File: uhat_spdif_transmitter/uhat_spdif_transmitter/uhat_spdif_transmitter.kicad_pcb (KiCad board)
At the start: 2 copper layers, 65 x 30 mm, 75 parts, among them J1 GPIO_CONNECTOR, Q1 SS8050, SW1 SW_Push, U1 PLT131/T8, U10 USBLC6-2SC6, U2 LR8103A-T12, U4 W25Q32JVSSIQ, U5 24LC256T-I/SN, U6 PLT131/T8, U8 ICE40UP5K-SG48I, X1 1651-24575-BTBEYA

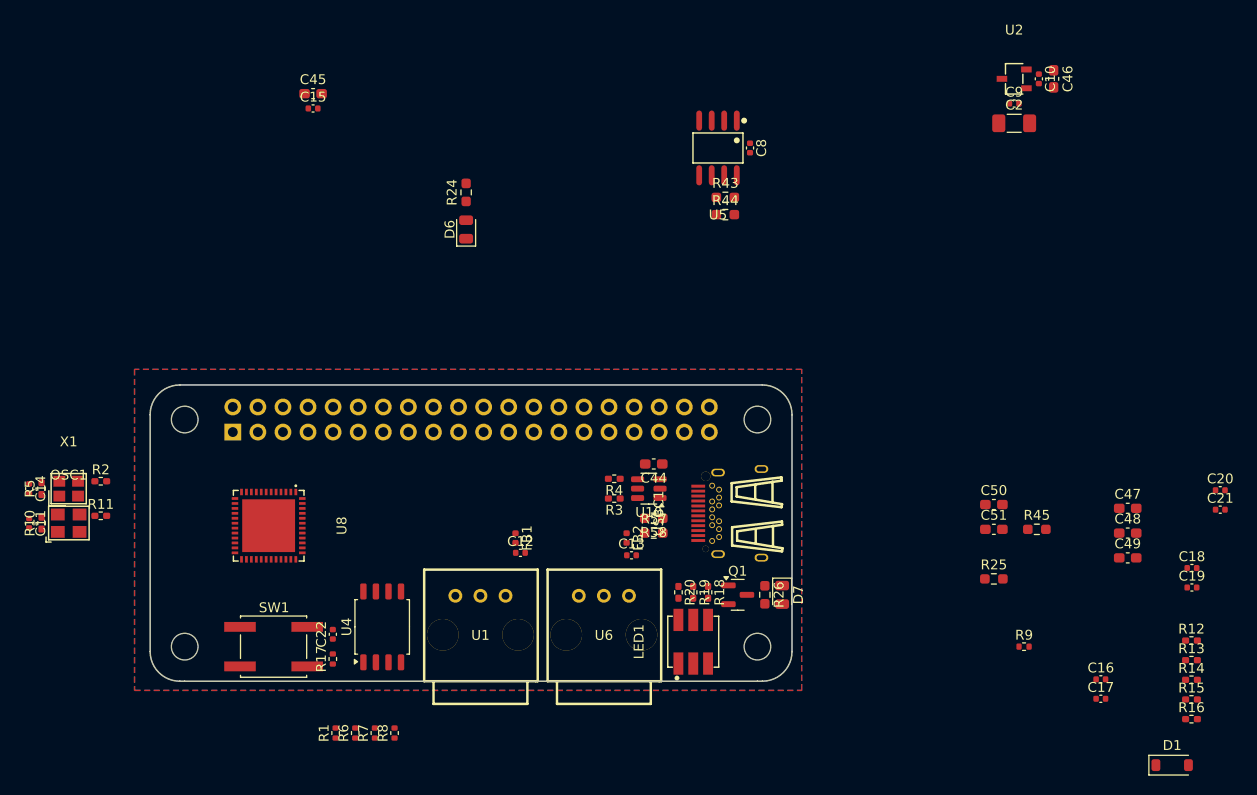
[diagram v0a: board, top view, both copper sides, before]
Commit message: layout
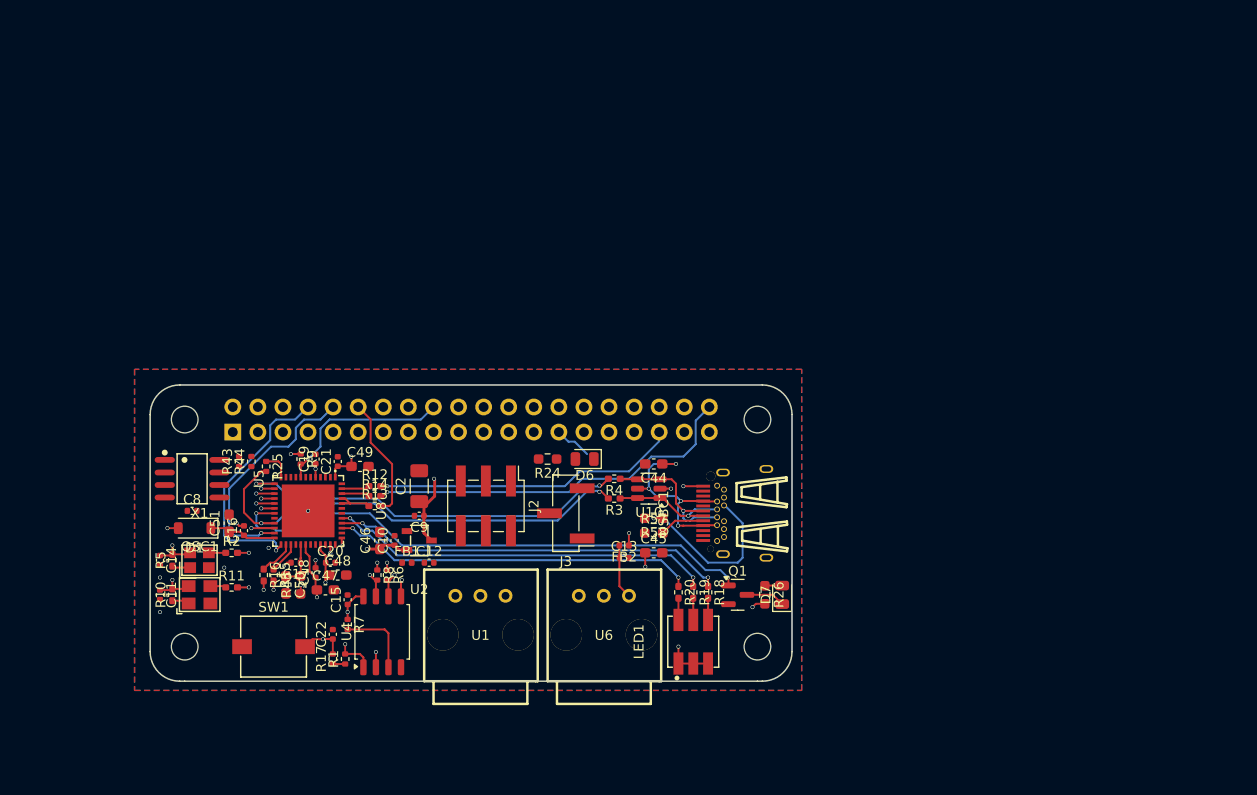
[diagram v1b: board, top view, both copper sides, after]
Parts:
- added J2: Conn_02x03_Odd_Even, Connector_PinHeader_2.54mm:PinHeader_2x03_P2.54mm_Vertical_SMD, F.Cu at (151.5, 103.3)
- added J3: Conn_01x03_Pin, Connector_PinHeader_2.54mm:PinHeader_1x03_P2.54mm_Vertical_SMD_Pin1Left, F.Cu at (159.6, 104.1)
- added REF**: Raspberry Pi Zero 2 W, Locrius_KiCad:Raspberry Pi Zero 2 W, F.Cu at (149.8, 106.1)
- R25, R43, R44: footprint Resistor_SMD:R_0603_1608Metric_Pad0.98x0.95mm_HandSolder -> Resistor_SMD:R_0402_1005Metric
- R3, R4: value 27R -> 68R
- SW1: value SW_Push -> SPEH110100; footprint Button_Switch_SMD:SW_SPST_EVQQ2 -> Locrius_KiCad:SW-SMD_L6.0-W6.0-LS6.6
- moved D1 101.9 mm to (122.0, 105.6), turned to 180 degrees
- moved R16 95.1 mm to (129.0, 110.3), turned to -90 degrees
- moved R15 93.8 mm to (130.0, 110.3), turned to -90 degrees
- moved C20 90.4 mm to (135.8, 109.1)
- moved C19 89.7 mm to (134.3, 98.6), turned to 90 degrees
- moved C21 89.5 mm to (136.5, 98.8), turned to 90 degrees
- moved C18 88.8 mm to (134.3, 110.1), turned to 90 degrees
- moved C16 88.1 mm to (127.0, 105.8), turned to 90 degrees
- moved R14 84.8 mm to (140.3, 102.3)
- moved R12 84.2 mm to (140.3, 101.3)
- moved R13 84.2 mm to (140.3, 103.3)
- moved C46 82.7 mm to (140.8, 106.8), turned to 90 degrees
- moved C17 82.7 mm to (132.3, 109.1), turned to 180 degrees
- moved C47 81.7 mm to (135.3, 111.8)
- moved C10 80.3 mm to (142.3, 106.8), turned to 90 degrees
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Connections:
- net /DM renamed /DN
- R12 pad 2: /PCM_FCLK -> /FPGA_FCLK
- R13 pad 2: /PCM_BCLK -> /FPGA_BCLK
- R14 pad 2: /PCM_DOUT -> /FPGA_DOUT
- U8 pad 10: /QSPI_SD2 -> unconnected-(U8-IOB_18a-Pad10)
- U8 pad 14: /QSPI_SD0 -> /SPI_MOSI
- U8 pad 15: /QSPI_SCLK -> /SPI_SCK
- U8 pad 16: /QSPI_SS -> /SPI_SS
- U8 pad 17: /QSPI_SD1 -> /SPI_MISO
- U8 pad 20: /QSPI_SD3 -> unconnected-(U8-IOB_25b_G3-Pad20)
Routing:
- net /USER_LED: track 0.00 -> 55.3 mm, vias 0 -> 2
- net /DP: track 0.00 -> 47.2 mm, vias 0 -> 2
- net +3V3: track 0.00 -> 42.2 mm, vias 0 -> 15
- net /DN: track 0.00 -> 40.6 mm, vias 0 -> 2
- net /RGB1: track 0.00 -> 40.3 mm, vias 0 -> 2
- net /RGB2: track 0.00 -> 39.0 mm, vias 0 -> 2
- net /PCM_DOUT: track 0.00 -> 38.4 mm, vias 0 -> 1
- net /RGB0: track 0.00 -> 37.1 mm, vias 0 -> 2
- net /PCM_FCLK: track 0.00 -> 31.0 mm, vias 0 -> 1
- net /UART_TX: track 0.00 -> 24.8 mm, vias 0 -> 1
- net /UART_RX: track 0.00 -> 23.8 mm, vias 0 -> 1
- net Net-(U10-VBUS): track 0.00 -> 21.5 mm, vias 0 -> 4
- net /CRESET: track 0.00 -> 18.2 mm, vias 0 -> 1
- net Net-(USBC1-CC2): track 0.00 -> 18.1 mm, vias 0 -> 1
- net /D-: track 0.00 -> 14.8 mm, vias 0 -> 1
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- added copper zone on In1.Cu, net +1V2
- added copper zone on In1.Cu, net +3V3
- added copper zone on In2.Cu, net GND
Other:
- copper layers 2 -> 4
